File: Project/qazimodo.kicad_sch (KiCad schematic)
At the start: 21 parts, among them J2 Conn_01x04_MountingPin, J3 USB_C_Receptacle_USB2.0, SW2 SW_push, U1 STM32F072CBTx

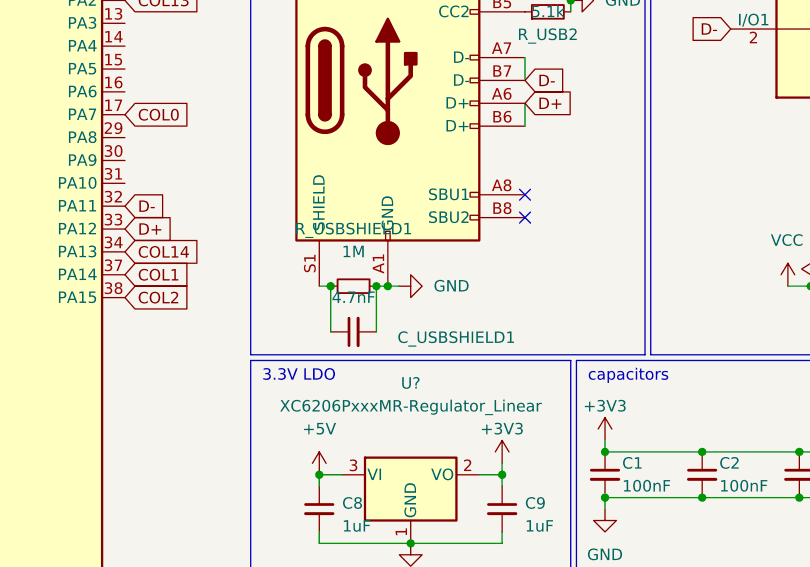
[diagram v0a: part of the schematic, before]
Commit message: revision wip
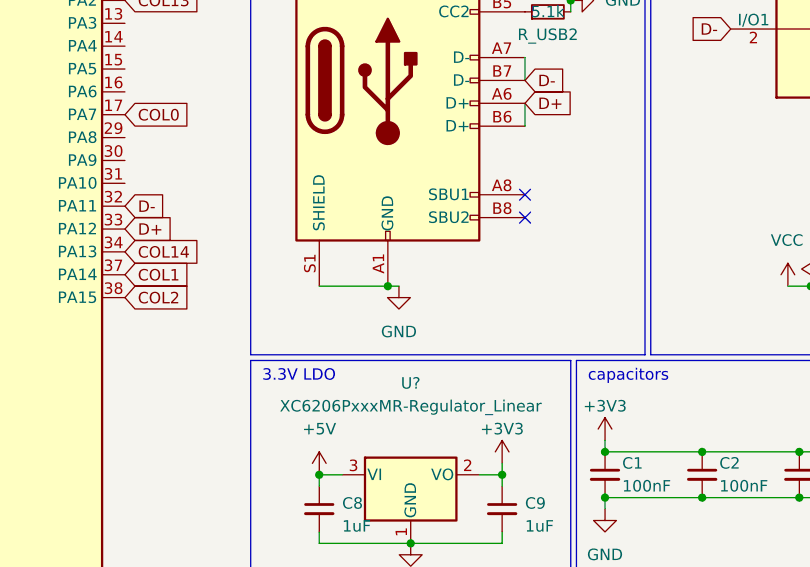
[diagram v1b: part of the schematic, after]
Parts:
- removed C_USBSHIELD1: 4.7nF, Capacitor_SMD:C_0402_1005Metric, symbol Device:C_Small
- removed R_USBSHIELD1: 1M, Resistor_SMD:R_0402_1005Metric, symbol Device:R_Small
- C1, C2, C3, C4, C5, C6, C7, C8, C9: footprint Capacitor_SMD:C_0402_1005Metric -> Capacitor_SMD:C_0805_2012Metric_Pad1.18x1.45mm_HandSolder
- D72: footprint Package_TO_SOT_SMD:SOT-143 -> Package_TO_SOT_SMD:SOT-143_Handsoldering
- F1: footprint Fuse:Fuse_1206_3216Metric -> Fuse:Fuse_1206_3216Metric_Pad1.42x1.75mm_HandSolder
- R1, R_USB1, R_USB2: footprint Resistor_SMD:R_0402_1005Metric -> Resistor_SMD:R_0805_2012Metric_Pad1.20x1.40mm_HandSolder
- U?: footprint Package_TO_SOT_SMD:SOT-23 -> Package_TO_SOT_SMD:SOT-23_Handsoldering
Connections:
- net GND: now also J3.S1 (SHIELD)
